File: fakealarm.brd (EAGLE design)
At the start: 28.1 x 34 mm, 17 parts, among them IC1 NE555N, Q1 2N3904, X1 RUN, X2 BAT, X3 GND, X4 +, X5 LED

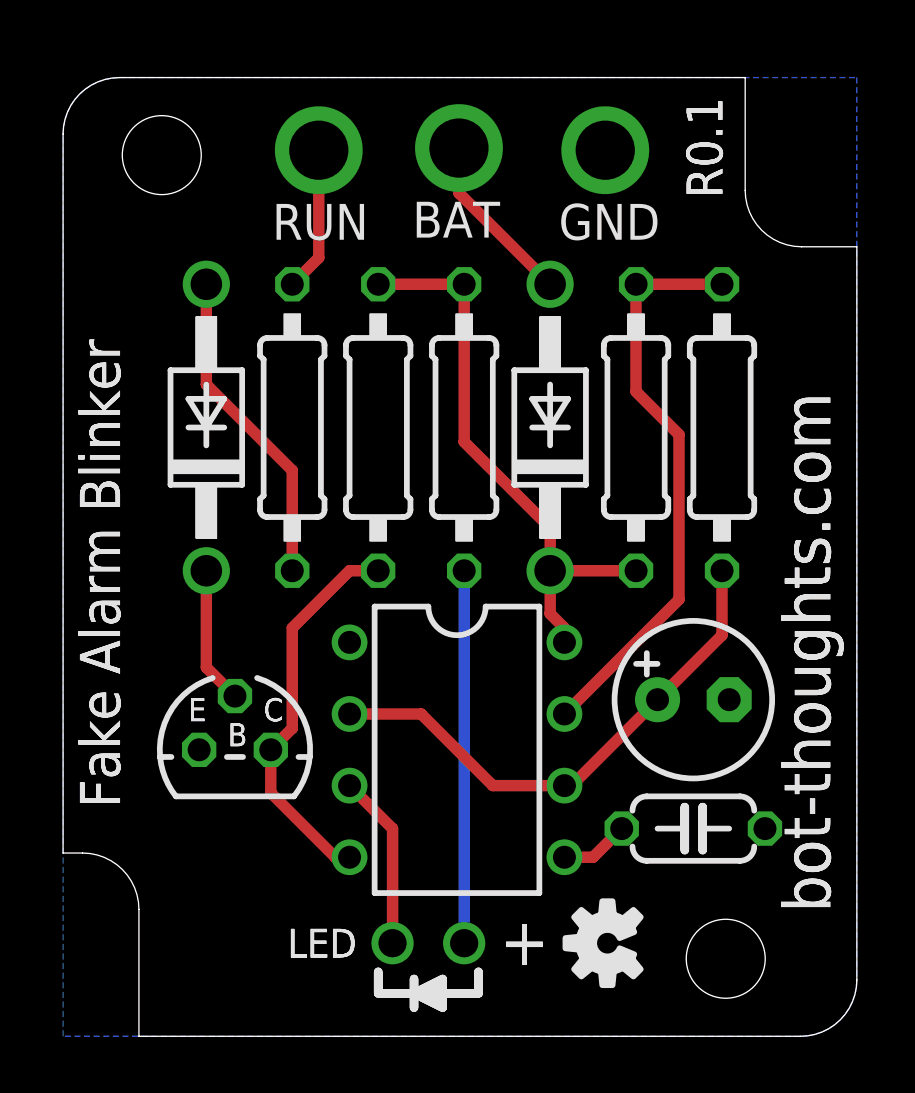
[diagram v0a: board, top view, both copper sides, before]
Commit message: Revised switch to use two mosfets to switch entire 555, revised layout, silk, added enclosure info to board
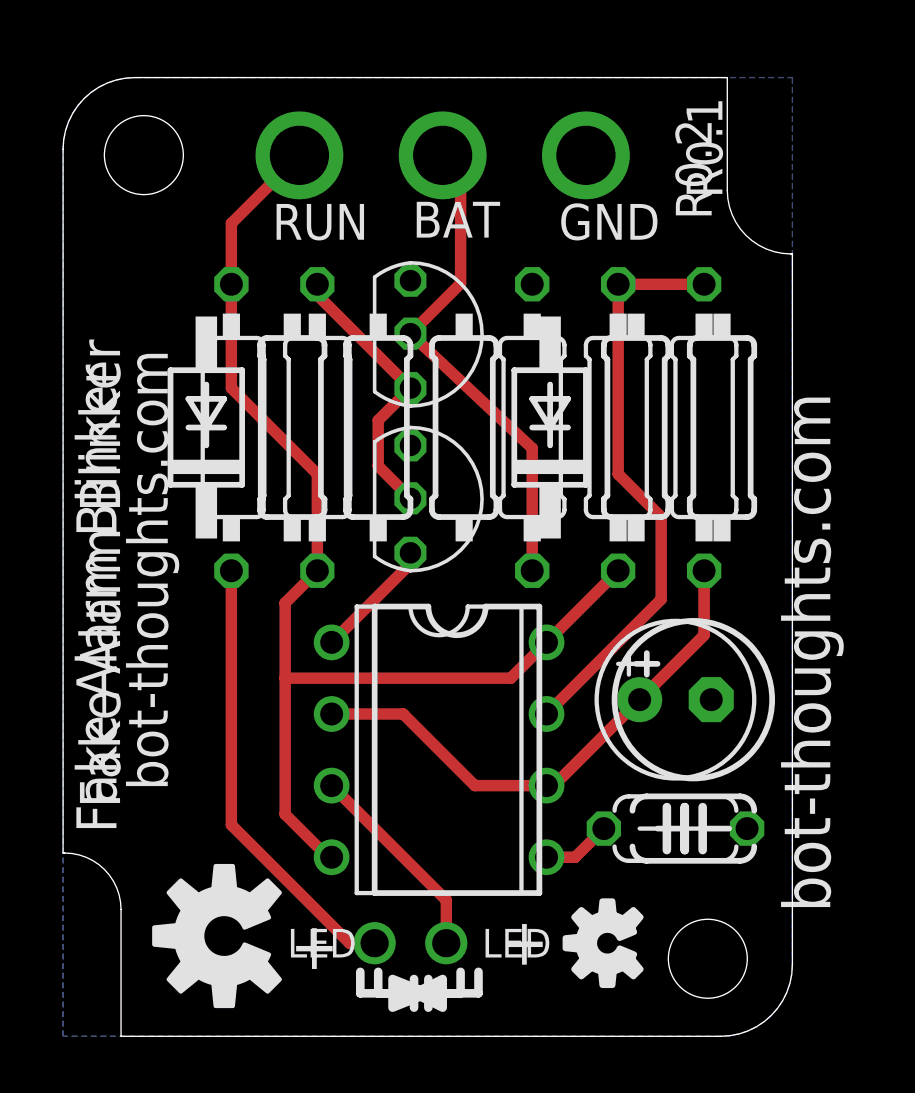
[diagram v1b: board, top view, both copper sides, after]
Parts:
- removed D1, D2: 1N4004, diode:DO41-10
- added Q2: 2N7000, ads4:TO92D-
- IC1: value NE555N -> LTC555
- LOGO1: value OSHW-LOGOS -> OSHW-LOGOM; device SparkFun-Aesthetics:OSHW-LOGO-S -> SparkFun-Aesthetics:OSHW-LOGO-M
- Q1: value 2N3904 -> 2N7000; device bt_transistor:TO92 -> ads4:TO92D-
- R3: value 1K -> 10k
- R4: value 100K -> 10k
- moved Q1 16.0 mm to (12.3, 24.9), turned to 270 degrees
- moved LOGO1 13.6 mm to (5.71, 3.56)
- moved R3 8.51 mm to (16.6, 21.6)
- moved R5 8.25 mm to (5.97, 21.6)
- moved X2 5.66 mm to (8.38, 31.2)
- moved X1 4.40 mm to (13.5, 31.2)
- moved X4 3.18 mm to (11.0, 3.30), turned to 180 degrees
- moved R4 2.16 mm to (9.02, 21.6), turned to 90 degrees
- moved X5 1.91 mm to (13.6, 3.30), turned to 0 degrees
- moved X3 0.71 mm to (18.5, 31.2)
- moved C1 0.64 mm to (21.7, 11.9)
- moved C2 0.64 mm to (21.7, 7.37)
- moved R1 0.64 mm to (19.7, 21.6)
- moved IC1 0.63 mm to (13.3, 10.2)
- moved R2 0.63 mm to (22.7, 21.6)
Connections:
- removed net N$11: IC1.4, Q1.1, R4.2
- removed net N$6: D2.A, X2.P$1
- net 12V: now also IC1.4, X2.P$1; no longer D2.C
- net GND: now also Q1.1, Q2.1, R3.2; no longer IC1.1, Q1.3
- net N$1: now also Q1.3, Q2.2, R4.2; no longer D1.A, R3.1
- net N$2: now also R3.1, X1.P$1; no longer D1.C
- net N$5: now also IC1.1, Q2.3; no longer R3.2, X1.P$1
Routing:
- net 12V: track 20.3 -> 41.8 mm
- net N$11: track 13.8 -> 0.00 mm
- net N$2: track 4.87 -> 17.6 mm
- net N$6: track 6.17 -> 0.00 mm
- net N$9: track 13.2 -> 15.8 mm
- net N$1: track 11.4 -> 9.91 mm
- net N$10: track 6.22 -> 7.27 mm
- net N$5: track 5.14 -> 4.59 mm
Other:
- board size 28.1 x 34 mm -> 25.9 x 34 mm
- board text added: "R0.2"
- board text removed: "2N3904"
- board text removed: "B"
- board text removed: "C"
- board text removed: "E"
